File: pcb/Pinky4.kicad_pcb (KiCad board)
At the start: 2 copper layers, 139 x 120 mm, 80 parts, among them J1 MJ-4PP-9, P1 i2c-pin, P2 i2c-pin, SW1 RESET_SW, SW10 SW_PUSH, SW11 SW_PUSH, SW12 SW_PUSH, SW13 SW_PUSH, SW14 SW_PUSH, SW15 SW_PUSH, SW16 SW_PUSH, SW17 SW_PUSH, SW18 SW_PUSH, SW19 SW_PUSH, SW2 SW_PUSH, SW20 SW_PUSH, SW21 SW_PUSH, SW22 SW_PUSH, SW23 SW_PUSH, SW24 SW_PUSH, SW25 SW_PUSH, SW26 SW_PUSH, SW27 SW_PUSH, SW28 SW_PUSH, SW29 SW_PUSH, SW3 SW_PUSH, SW30 SW_PUSH, SW31 SW_PUSH, SW32 SW_PUSH, SW33 SW_PUSH, SW4 SW_PUSH, SW5 SW_PUSH, SW6 SW_PUSH, SW7 SW_PUSH, SW8 SW_PUSH, SW9 SW_PUSH, U1 ProMicro

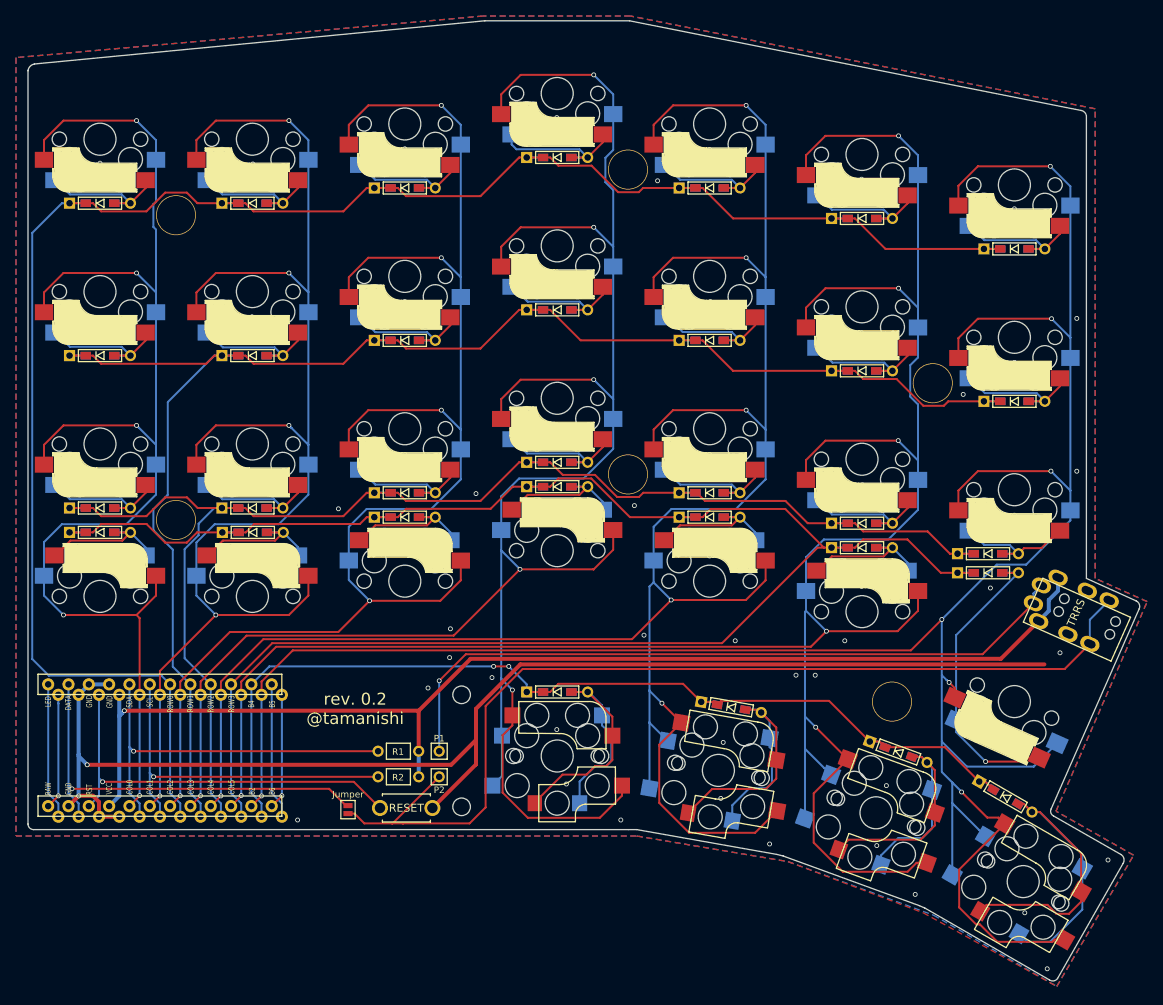
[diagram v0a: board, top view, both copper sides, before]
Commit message: - readme - rename to Pinky4
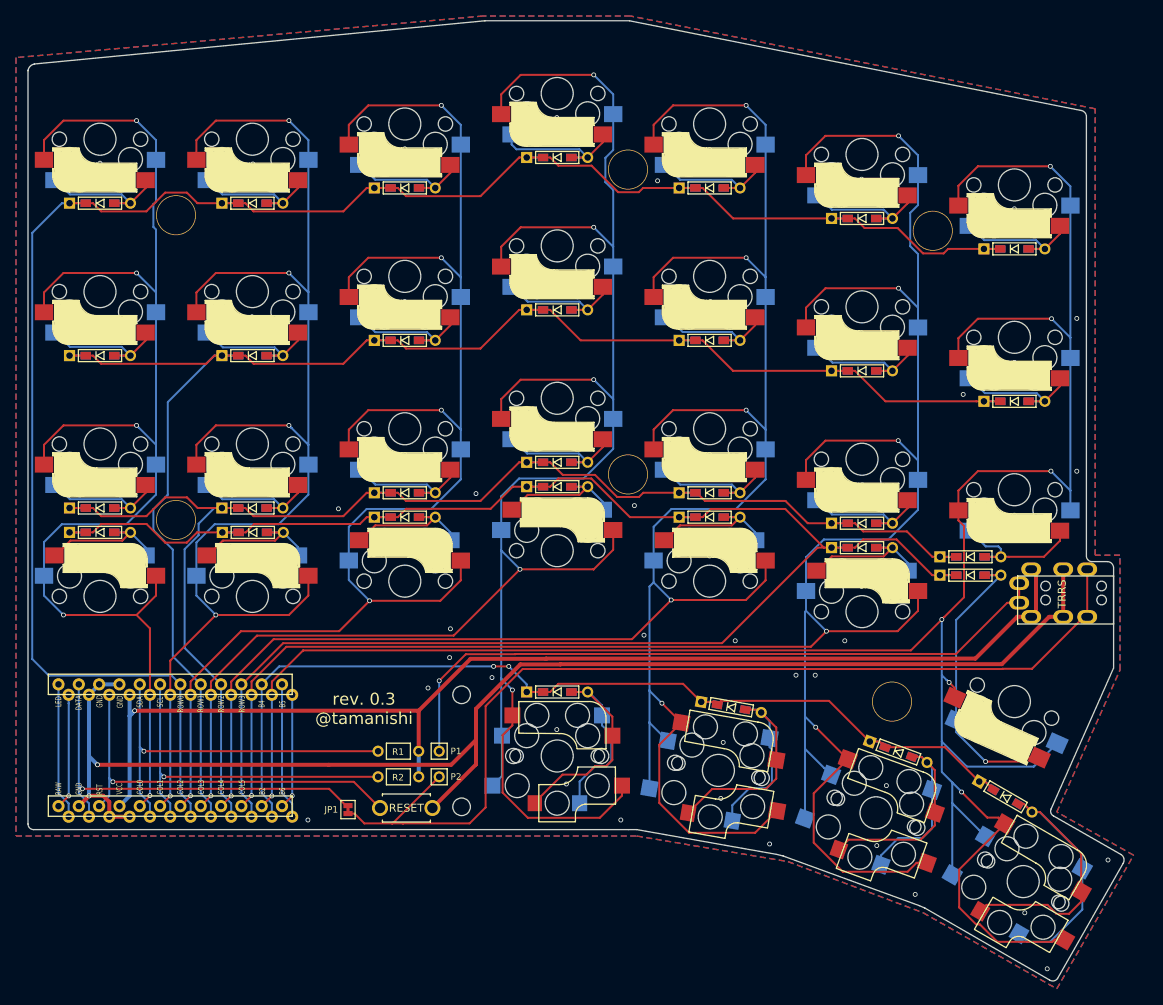
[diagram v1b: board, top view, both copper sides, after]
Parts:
- JP1: value Jumper -> JP; footprint kbd:Jumper -> kbd:JP
- moved Ref** 19.0 mm to (154.1, 61.5)
- moved J1 4.98 mm to (176.7, 107.6), turned to 270 degrees
- moved D30 2.23 mm to (158.8, 102.2)
- moved D31 2.22 mm to (158.8, 104.5)
- moved U1 1.29 mm to (59.3, 125.8)
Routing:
- net GND: track 165.7 -> 175.2 mm, vias 60 -> 58
- net col6: track 318.1 -> 309.4 mm
- net row3: track 236.8 -> 233.3 mm
- net VCC: track 149.0 -> 147.1 mm
- net Net-(J1-PadA): track 89.7 -> 87.8 mm
- net row2: track 181.7 -> 179.9 mm
- net Net-(D30-Pad2): track 17.9 -> 19.6 mm
- net row0: track 236.8 -> 238.6 mm
- net col3: track 268.1 -> 266.8 mm
- net col2: track 185.4 -> 184.1 mm
- net reset: track 51.1 -> 49.8 mm
- net sda: track 48.4 -> 47.1 mm
- net scl: track 45.8 -> 44.5 mm
- net data: track 53.0 -> 51.8 mm
- net col5: track 300.7 -> 299.4 mm
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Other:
- board size 139 x 120 mm -> 137 x 120 mm
- board text added: "rev. 0.3 @tamanishi"
- board text removed: "rev. 0.2 @tamanishi"
